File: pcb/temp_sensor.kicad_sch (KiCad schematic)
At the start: 4 parts, among them SW3 PTS810

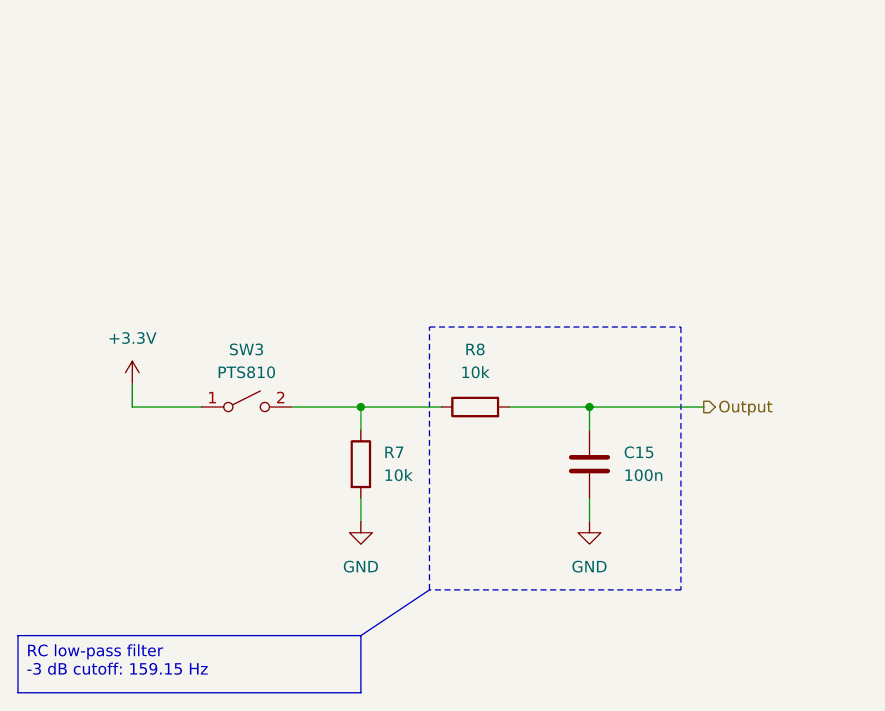
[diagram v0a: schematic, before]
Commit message: add top level schem and cleanup
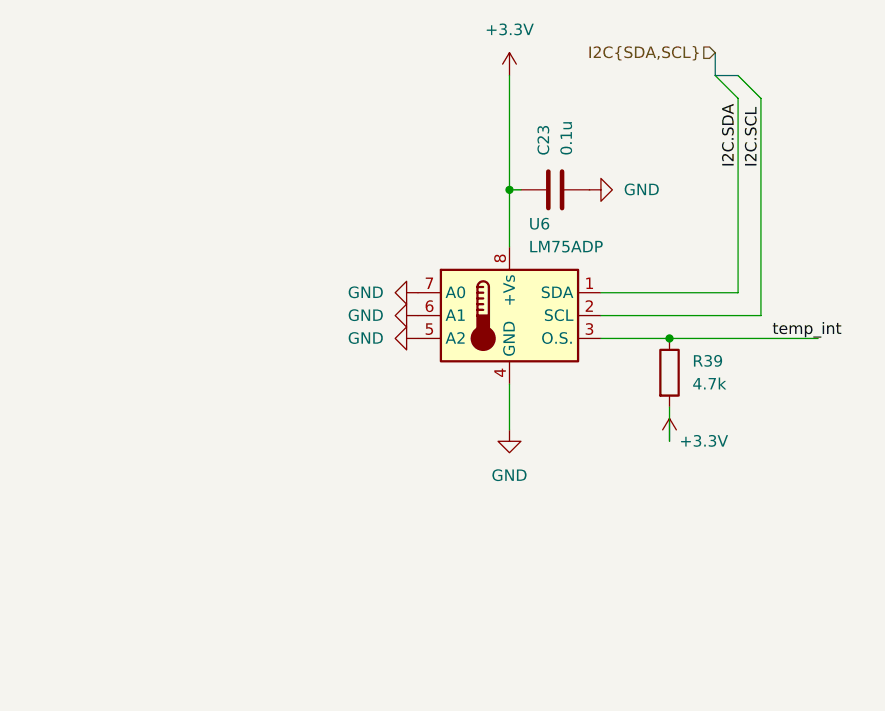
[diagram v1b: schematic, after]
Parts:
- removed C15: 100n, Capacitor_SMD:C_0402_1005Metric, symbol Device:C
- removed R7, R8: 10k, Resistor_SMD:R_0402_1005Metric, symbol Device:R
- removed SW3: PTS810, Button_Switch_SMD:SW_SPST_PTS810, symbol Switch:SW_SPST
- added C23: 0.1u, symbol Device:C
- added R39: 4.7k, symbol Device:R
- added U6: LM75ADP, symbol Sensor_Temperature:LM75B
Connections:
- net +3.3V: now also C23.1, R39.2, U6.8 (+Vs)
- net GND: now also C23.2, U6.4 (GND), U6.5 (A2), U6.6 (A1), U6.7 (A0)
- new net I2C.SCL: U6.2 (SCL)
- new net I2C.SDA: U6.1 (SDA)
- new net temp_int: R39.1, U6.3 (O.S.)
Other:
- company: RoboJackets Electrical Training -> (none)
- title: Debounced Button -> Temperature Sensor
